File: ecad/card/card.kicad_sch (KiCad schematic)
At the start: 53 parts, among them J1 Conn_01x03_Pin, J2 USB4105-GF-A, J3 10145226-0241N13LF, SW1 SW_Push, SW2 SW_Push, U1 W25Q128JVS, U2 RP2350_80QFN, U3 MCP23017_SO, U4 NCP1117-3.3_SOT223, U5 MCP23017_SO, X1 ABM8-272-T3

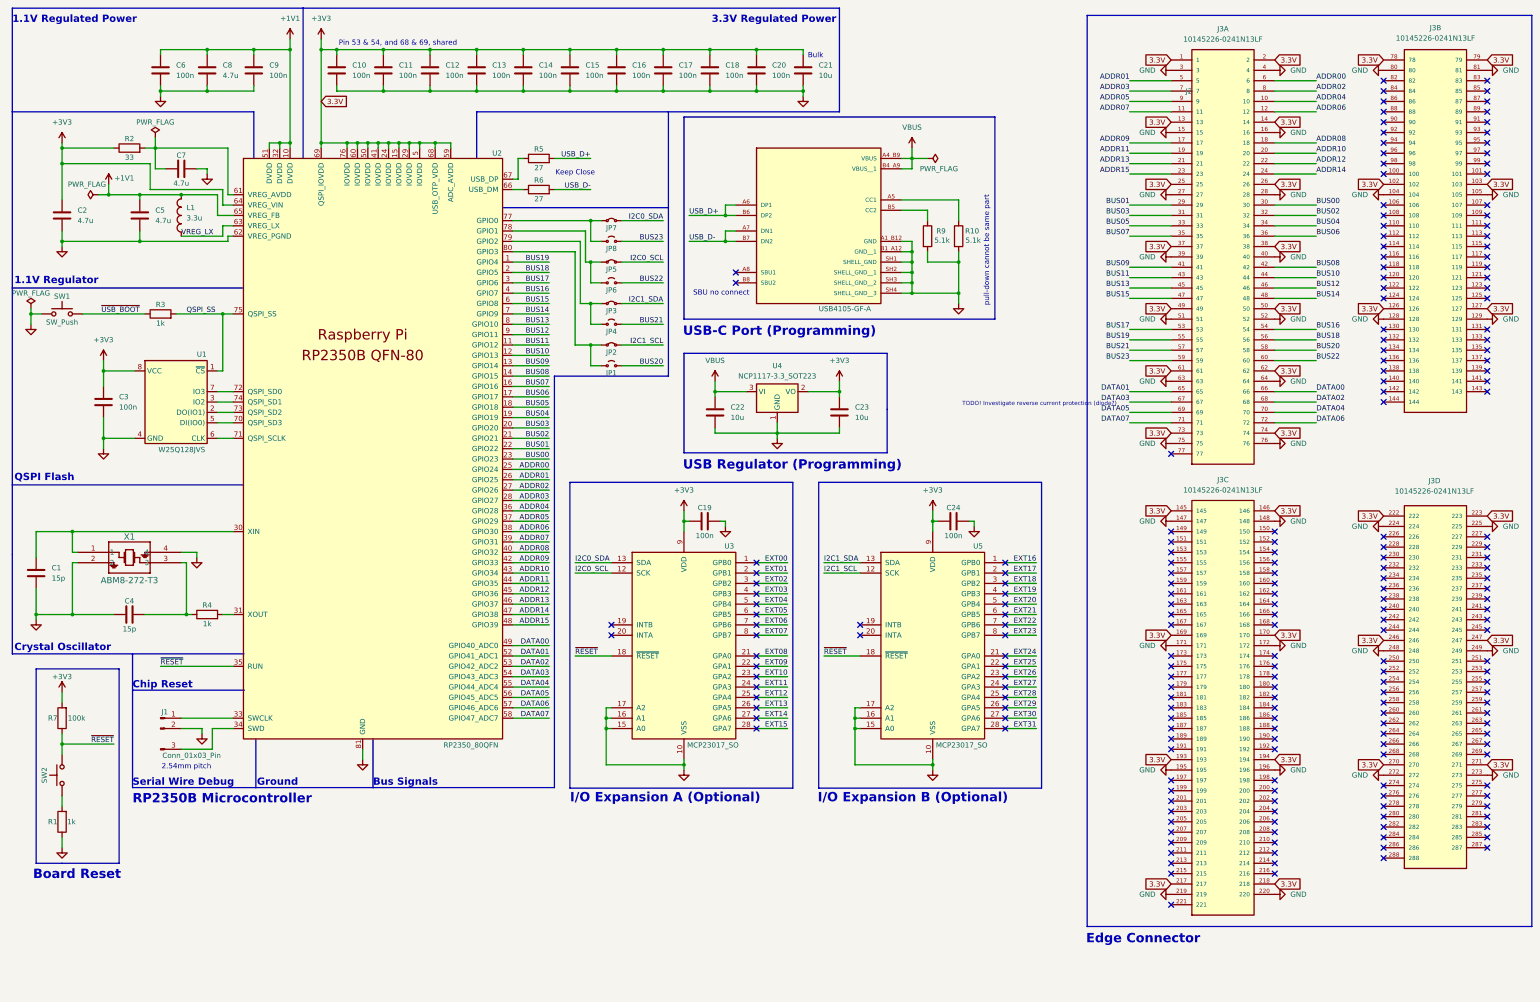
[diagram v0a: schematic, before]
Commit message: near-final card layout
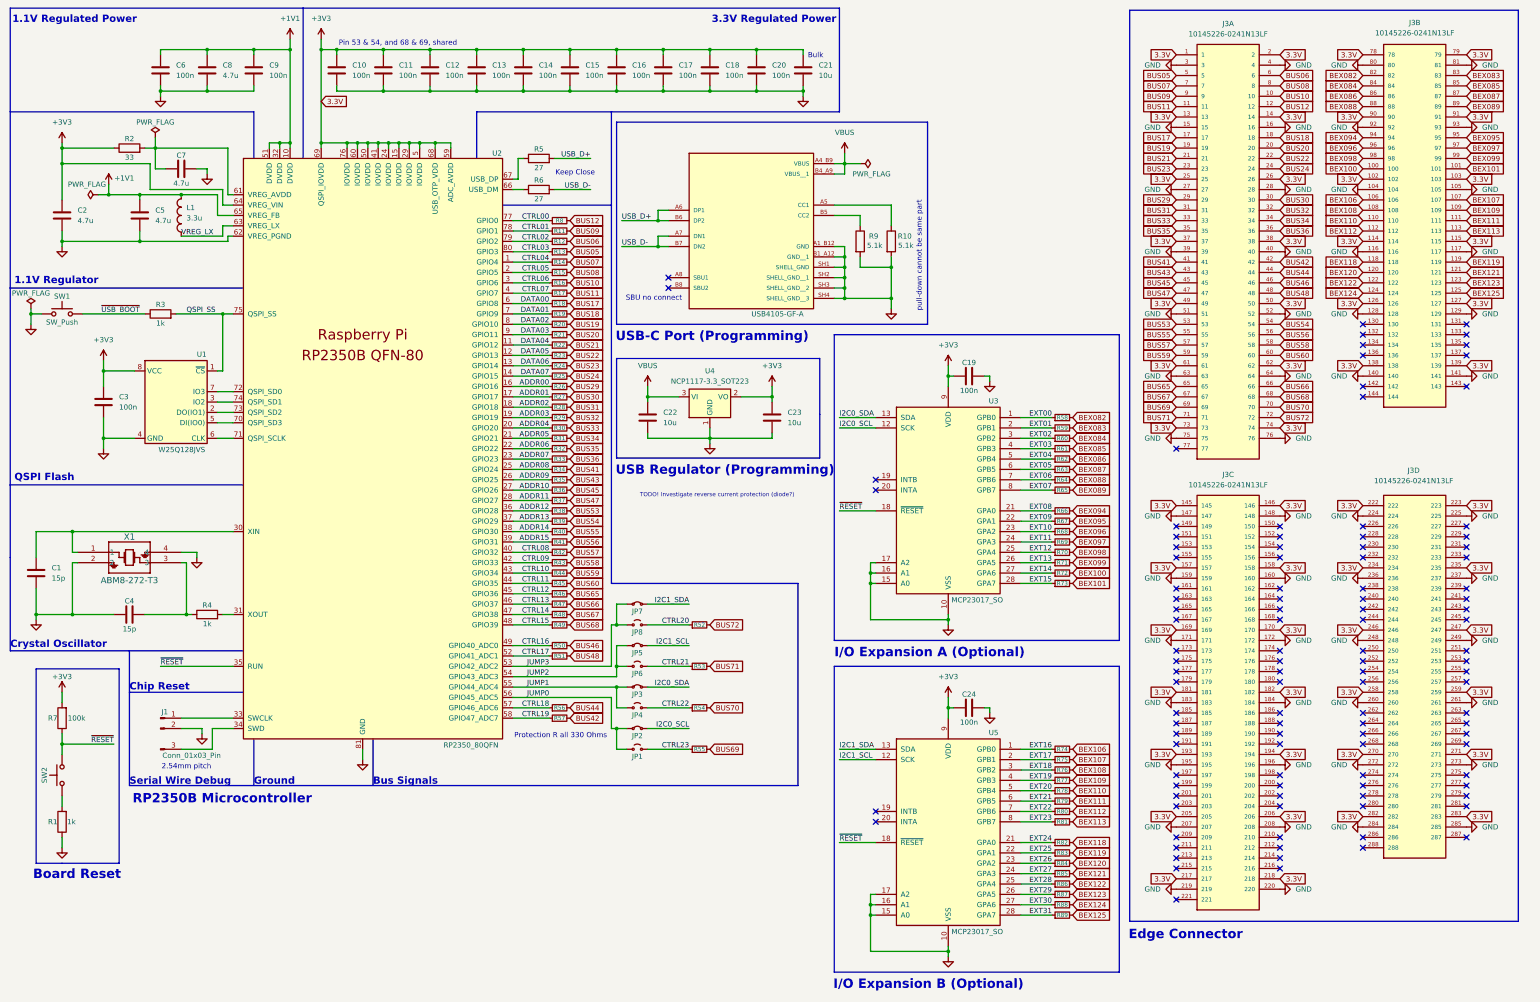
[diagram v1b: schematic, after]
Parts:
- added R11, R12, R13, R14, R15, R16, R17, R18, R19, R20, R21, R22, R23, R24, R25, R26, R27, R28, R29, R30, R31, R32, R33, R34, R35, R36, R37, R38, R39, R40, R41, R42, R43, R44, R45, R46, R47, R48, R49, R50, R51, R52, R53, R54, R55, R56, R57, R58, R59, R60, R61, R62, R63, R64, R65, R66, R67, R68, R69, R70, R71, R72, R73, R74, R75, R76, R77, R78, R79, R8, R80, R81, R82, R83, R84, R85, R86, R87, R88, R89: 330, Resistor_SMD:R_0402_1005Metric, symbol Device:R_Small
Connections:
- net +3V3: now also J3.114, J3.115, J3.138, J3.139, J3.157, J3.158, J3.181, J3.182, J3.205, J3.206, J3.234, J3.235, J3.258, J3.259, J3.282, J3.283, J3.90, J3.91
- net ADDR00: now also U2.16 (GPIO16), R26.1; no longer J3.6, U2.25 (GPIO24)
- net ADDR01: now also U2.17 (GPIO17), R27.1; no longer J3.5, U2.26 (GPIO25)
- net ADDR02: now also U2.18 (GPIO18), R28.1; no longer J3.8, U2.27 (GPIO26)
- net ADDR03: now also U2.19 (GPIO19), R29.1; no longer J3.7, U2.28 (GPIO27)
- net ADDR04: now also U2.20 (GPIO20), R30.1; no longer J3.10, U2.36 (GPIO28)
- net ADDR05: now also U2.21 (GPIO21), R31.1; no longer J3.9, U2.37 (GPIO29)
- net ADDR06: now also U2.22 (GPIO22), R32.1; no longer J3.12, U2.38 (GPIO30)
- net ADDR07: now also U2.23 (GPIO23), R33.1; no longer J3.11, U2.39 (GPIO31)
- net ADDR08: now also U2.25 (GPIO24), R34.1; no longer J3.18, U2.40 (GPIO32)
- net ADDR09: now also U2.26 (GPIO25), R35.1; no longer J3.17, U2.42 (GPIO33)
- net ADDR10: now also U2.27 (GPIO26), R36.1; no longer J3.20, U2.43 (GPIO34)
- net ADDR11: now also U2.28 (GPIO27), R37.1; no longer J3.19, U2.44 (GPIO35)
- net ADDR12: now also U2.36 (GPIO28), R38.1; no longer J3.22, U2.45 (GPIO36)
- net ADDR13: now also U2.37 (GPIO29), R39.1; no longer J3.21, U2.46 (GPIO37)
- net ADDR14: now also U2.38 (GPIO30), R40.1; no longer J3.24, U2.47 (GPIO38)
- net ADDR15: now also U2.39 (GPIO31), R41.1; no longer J3.23, U2.48 (GPIO39)
- net BUS05: now also J3.5, R13.2; no longer J3.33, U2.18 (GPIO18)
- net BUS06: now also J3.6, R12.2; no longer J3.36, U2.17 (GPIO17)
- net BUS07: now also J3.7, R14.2; no longer J3.35, U2.16 (GPIO16)
- net BUS08: now also J3.8, R15.2; no longer J3.42, U2.14 (GPIO15)
- net BUS09: now also J3.9, R11.2; no longer J3.41, U2.13 (GPIO14)
- net BUS10: now also J3.10, R16.2; no longer J3.44, U2.12 (GPIO13)
- net BUS11: now also J3.11, R17.2; no longer J3.43, U2.11 (GPIO12)
- net BUS12: now also J3.12, R8.2; no longer J3.46, U2.9 (GPIO11)
- net BUS17: now also J3.17, R18.2; no longer J3.53, U2.3 (GPIO6)
- net BUS18: now also J3.18, R19.2; no longer J3.56, U2.2 (GPIO5)
- net BUS19: now also J3.19, R20.2; no longer J3.55, U2.1 (GPIO4)
- net BUS20: now also J3.20, R21.2; no longer J3.58, JP1.2 (B)
- net BUS21: now also J3.21, R22.2; no longer J3.57, JP4.2 (B)
- net BUS22: now also J3.22, R23.2; no longer J3.60, JP6.2 (B)
- net BUS23: now also J3.23, R24.2; no longer J3.59, JP8.2 (B)
- net DATA00: now also U2.6 (GPIO8), R18.1; no longer J3.66, U2.49 (GPIO40_ADC0)
- net DATA01: now also U2.7 (GPIO9), R19.1; no longer J3.65, U2.52 (GPIO41_ADC1)
- net DATA02: now also U2.8 (GPIO10), R20.1; no longer J3.68, U2.53 (GPIO42_ADC2)
- net DATA03: now also U2.9 (GPIO11), R21.1; no longer J3.67, U2.54 (GPIO43_ADC3)
- net DATA04: now also U2.11 (GPIO12), R22.1; no longer J3.70, U2.55 (GPIO44_ADC4)
- net DATA05: now also U2.12 (GPIO13), R23.1; no longer J3.69, U2.56 (GPIO45_ADC5)
- net DATA06: now also U2.13 (GPIO14), R24.1; no longer J3.72, U2.57 (GPIO46_ADC6)
- net DATA07: now also U2.14 (GPIO15), R25.1; no longer J3.71, U2.58 (GPIO47_ADC7)
- net EXT00: now also R58.1
- net EXT01: now also R59.1
- net EXT02: now also R60.1
- net EXT03: now also R61.1
- net EXT04: now also R62.1
- net EXT05: now also R63.1
- net EXT06: now also R64.1
- net EXT07: now also R65.1
- net EXT08: now also R66.1
- net EXT09: now also R67.1
- net EXT10: now also R68.1
- net EXT11: now also R69.1
- net EXT12: now also R70.1
- net EXT13: now also R71.1
- net EXT14: now also R72.1
- net EXT15: now also R73.1
- net EXT16: now also R74.1
- net EXT17: now also R75.1
- net EXT18: now also R76.1
- net EXT19: now also R77.1
- net EXT20: now also R78.1
- net EXT21: now also R79.1
- net EXT22: now also R80.1
- net EXT23: now also R81.1
- net EXT24: now also R82.1
- net EXT25: now also R83.1
- net EXT26: now also R84.1
- net EXT27: now also R85.1
- net EXT28: now also R86.1
- net EXT29: now also R87.1
- net EXT30: now also R88.1
- net EXT31: now also R89.1
- net GND: now also J3.116, J3.117, J3.140, J3.141, J3.159, J3.160, J3.183, J3.184, J3.207, J3.208, J3.236, J3.237, J3.260, J3.261, J3.284, J3.285, J3.92, J3.93
- net I2C0_SCL: now also JP2.2 (B); no longer JP5.2 (B)
- net I2C0_SDA: now also JP3.2 (B); no longer JP7.2 (B)
- net I2C1_SCL: now also JP5.2 (B); no longer JP2.2 (B)
- net I2C1_SDA: now also JP7.2 (B); no longer JP3.2 (B)
- net JUMP1: now reaches JP3.1 (A), JP4.1 (A)
- net JUMP1: now also U2.55 (GPIO44_ADC4); no longer U2.79 (GPIO2)
- net JUMP3: now reaches JP7.1 (A), JP8.1 (A)
- net JUMP3: now also U2.53 (GPIO42_ADC2); no longer U2.77 (GPIO0)
- net JUMP2: now reaches JP5.1 (A), JP6.1 (A)
- net JUMP2: now also U2.54 (GPIO43_ADC3); no longer U2.78 (GPIO1)
- net JUMP0: now reaches JP1.1 (A), JP2.1 (A)
- net JUMP0: now also U2.56 (GPIO45_ADC5); no longer U2.80 (GPIO3)
- net BEX100: now reaches J3.100
- net BEX100: now also R72.2
- net BEX101: now reaches J3.101
- net BEX101: now also R73.2
- net BEX106: now reaches J3.106
- net BEX106: now also R74.2
- net BEX107: now reaches J3.107
- net BEX107: now also R75.2
- net BEX108: now reaches J3.108
- net BEX108: now also R76.2
- net BEX109: now reaches J3.109
- net BEX109: now also R77.2
- net BEX110: now reaches J3.110
- net BEX110: now also R78.2
- net BEX111: now reaches J3.111
- net BEX111: now also R79.2
- net BEX112: now reaches J3.112
- net BEX112: now also R80.2
- net BEX113: now reaches J3.113
- net BEX113: now also R81.2
- net BEX118: now reaches J3.118
- net BEX118: now also R82.2
- net BEX119: now reaches J3.119
- net BEX119: now also R83.2
- net BEX120: now reaches J3.120
- net BEX120: now also R84.2
- net BEX121: now reaches J3.121
- net BEX121: now also R85.2
- net BEX122: now reaches J3.122
- net BEX122: now also R86.2
- net BEX123: now reaches J3.123
- net BEX123: now also R87.2
- net BEX124: now reaches J3.124
- net BEX124: now also R88.2
- net BEX125: now reaches J3.125
- net BEX125: now also R89.2
- net BEX082: now reaches J3.82
- net BEX082: now also R58.2
- net BEX083: now reaches J3.83
- net BEX083: now also R59.2
- net BEX084: now reaches J3.84
- net BEX084: now also R60.2
- net BEX085: now reaches J3.85
- net BEX085: now also R61.2
- net BEX086: now reaches J3.86
- net BEX086: now also R62.2
- net BEX087: now reaches J3.87
- net BEX087: now also R63.2
- net BEX088: now reaches J3.88
- net BEX088: now also R64.2
- net BEX089: now reaches J3.89
- net BEX089: now also R65.2
- net BEX094: now reaches J3.94
- net BEX094: now also R66.2
- net BEX095: now reaches J3.95
- net BEX095: now also R67.2
- net BEX096: now reaches J3.96
- net BEX096: now also R68.2
- net BEX097: now reaches J3.97
- net BEX097: now also R69.2
- net BEX098: now reaches J3.98
- net BEX098: now also R70.2
- net BEX099: now reaches J3.99
- net BEX099: now also R71.2
- net BUS00 renamed BUS30
- net BUS30: now also R27.2; no longer U2.23 (GPIO23)
- net BUS01 renamed BUS29
- net BUS29: now also R26.2; no longer U2.22 (GPIO22)
- net BUS02 renamed BUS32
- net BUS32: now also R29.2; no longer U2.21 (GPIO21)
- net BUS03 renamed BUS31
- net BUS31: now also R28.2; no longer U2.20 (GPIO20)
- net BUS04 renamed BUS34
- net BUS34: now also R31.2; no longer U2.19 (GPIO19)
- net BUS13 renamed BUS45
- net BUS45: now also R36.2; no longer U2.8 (GPIO10)
- net BUS14 renamed BUS48
- net BUS48: now also R51.2; no longer U2.7 (GPIO9)
- net BUS15 renamed BUS47
- net BUS47: now also R37.2; no longer U2.6 (GPIO8)
- net BUS16 renamed BUS54
- net BUS54: now also R39.2; no longer U2.4 (GPIO7)
- new net BUS24: J3.24, R25.2
- new net BUS33: J3.33, R30.2
- new net BUS35: J3.35, R32.2
- new net BUS36: J3.36, R33.2
- new net BUS41: J3.41, R34.2
- new net BUS42: J3.42, R57.2
- new net BUS43: J3.43, R35.2
- new net BUS44: J3.44, R56.2
- new net BUS46: J3.46, R50.2
- new net BUS53: J3.53, R38.2
- new net BUS55: J3.55, R40.2
- new net BUS56: J3.56, R41.2
- new net BUS57: J3.57, R42.2
- new net BUS58: J3.58, R43.2
- new net BUS59: J3.59, R44.2
- new net BUS60: J3.60, R45.2
- new net BUS65: J3.65, R46.2
- new net BUS66: J3.66, R47.2
- new net BUS67: J3.67, R48.2
- new net BUS68: J3.68, R49.2
- new net BUS69: J3.69, R55.2
- new net BUS70: J3.70, R54.2
- new net BUS71: J3.71, R53.2
- new net BUS72: J3.72, R52.2
- new net CTRL00: R8.1, U2.77 (GPIO0)
- new net CTRL01: R11.1, U2.78 (GPIO1)
- new net CTRL02: R12.1, U2.79 (GPIO2)
- new net CTRL03: R13.1, U2.80 (GPIO3)
- new net CTRL04: R14.1, U2.1 (GPIO4)
- new net CTRL05: R15.1, U2.2 (GPIO5)
- new net CTRL06: R16.1, U2.3 (GPIO6)
- new net CTRL07: R17.1, U2.4 (GPIO7)
- new net CTRL08: R42.1, U2.40 (GPIO32)
- new net CTRL09: R43.1, U2.42 (GPIO33)
- new net CTRL10: R44.1, U2.43 (GPIO34)
- new net CTRL11: R45.1, U2.44 (GPIO35)
- new net CTRL12: R46.1, U2.45 (GPIO36)
- new net CTRL13: R47.1, U2.46 (GPIO37)
- new net CTRL14: R48.1, U2.47 (GPIO38)
- new net CTRL15: R49.1, U2.48 (GPIO39)
- new net CTRL16: R50.1, U2.49 (GPIO40_ADC0)
- new net CTRL17: R51.1, U2.52 (GPIO41_ADC1)
- new net CTRL18: R56.1, U2.57 (GPIO46_ADC6)
- new net CTRL19: R57.1, U2.58 (GPIO47_ADC7)
- new net CTRL20: JP8.2 (B), R52.1
- new net CTRL21: JP6.2 (B), R53.1
- new net CTRL22: JP4.2 (B), R54.1
- new net CTRL23: JP1.2 (B), R55.1
- no-connect marks 210 -> 110
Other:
- note added: "Protection R all 330 Ohms"
- moved on the sheet: C19, C22, C23, C24, J3A, J3B, J3C, J3D, JP1, JP2, JP3, JP4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
